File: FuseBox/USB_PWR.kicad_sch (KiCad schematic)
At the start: 54 parts, among them J1 UJ31CHG2SMTTR, U1 TPS61040DBVR, U2 LT3030EFETRPBF

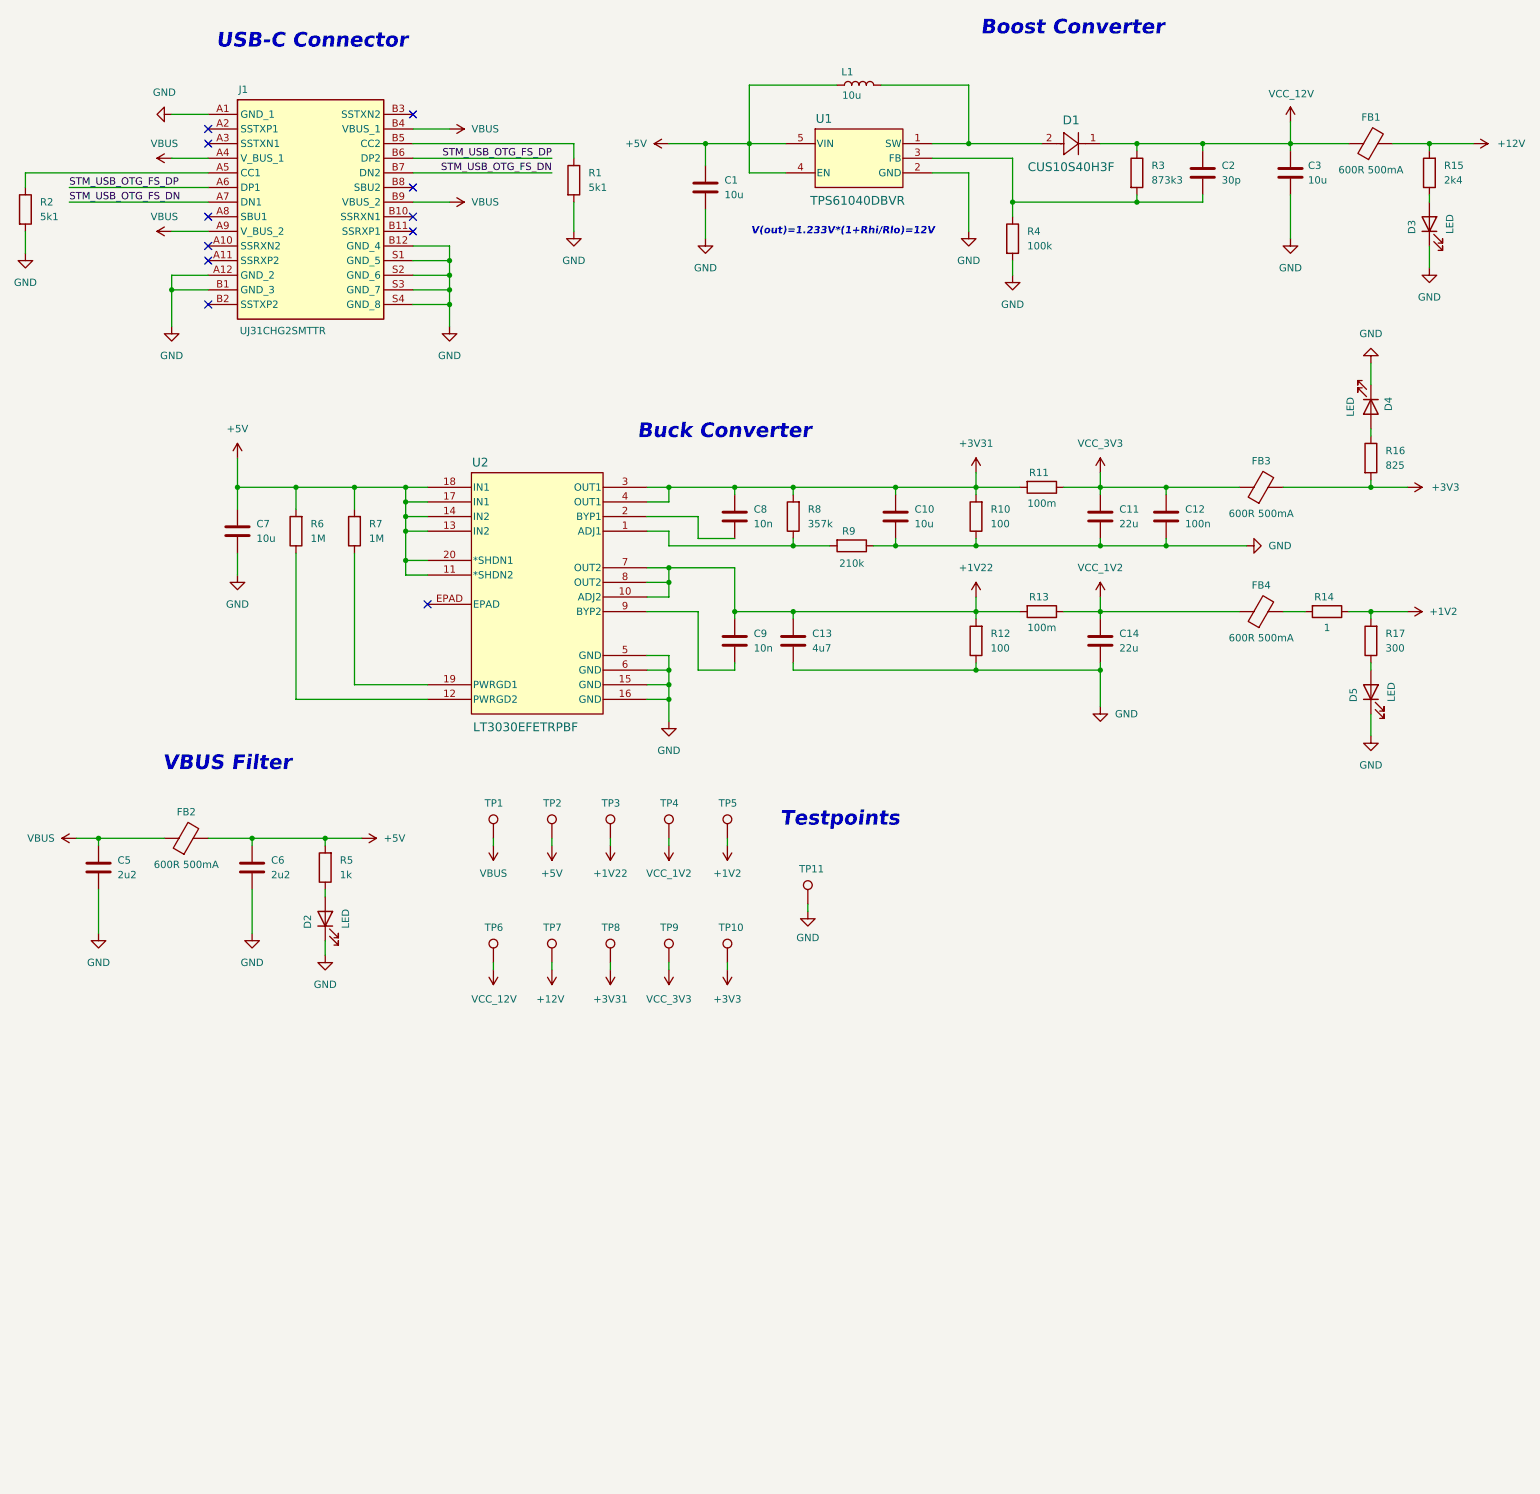
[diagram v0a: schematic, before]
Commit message: keeeek
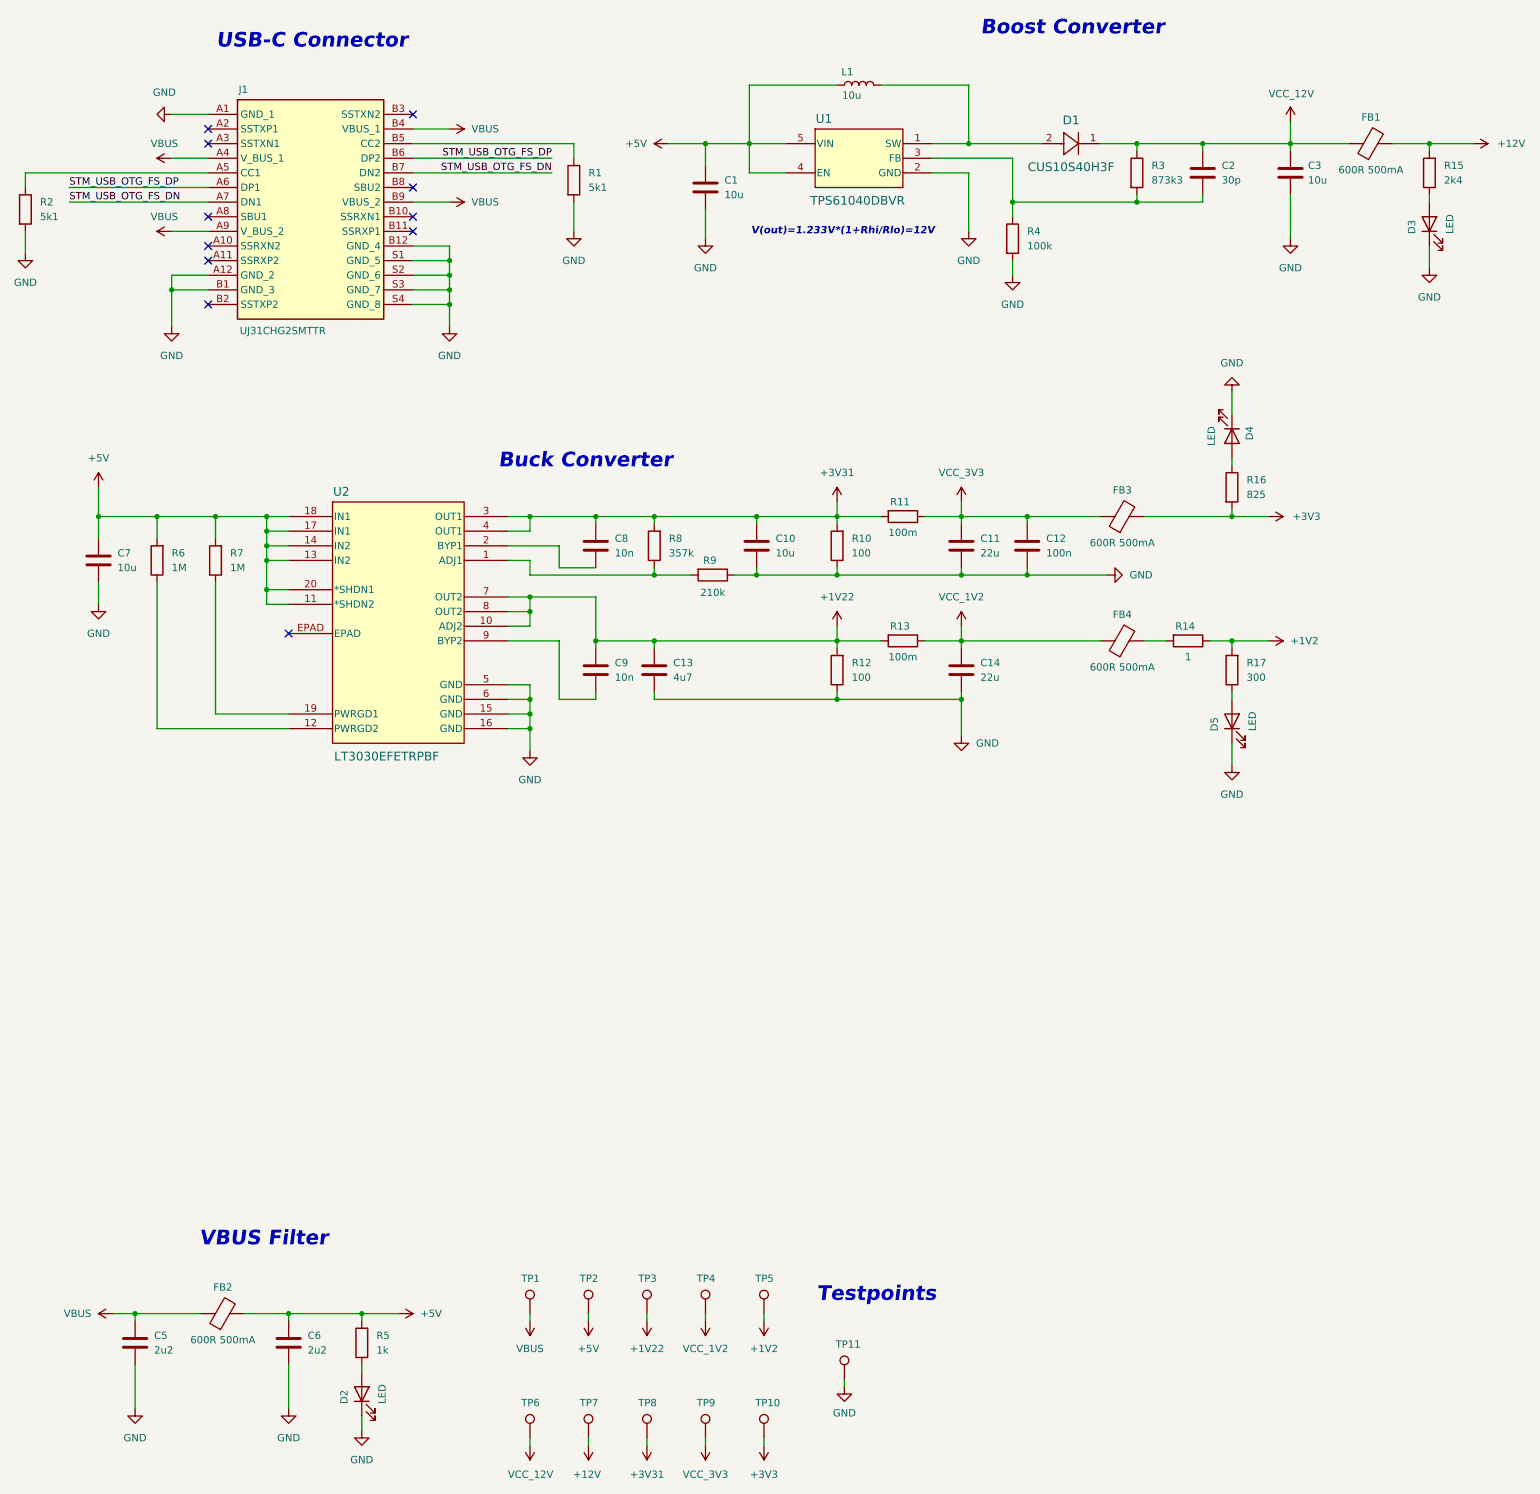
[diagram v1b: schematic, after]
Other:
- moved on the sheet: C10, C11, C12, C13, C14, C5, C6, C7, C8, C9, D2, D4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
